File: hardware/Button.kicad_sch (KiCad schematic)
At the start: 12 parts, among them J13 Conn_01x05_Pin, J5 Conn_01x05_Pin, Q1 2N7002, Q10 2N7002, Q2 2N7002, Q3 2N7002, Q9 2N7002

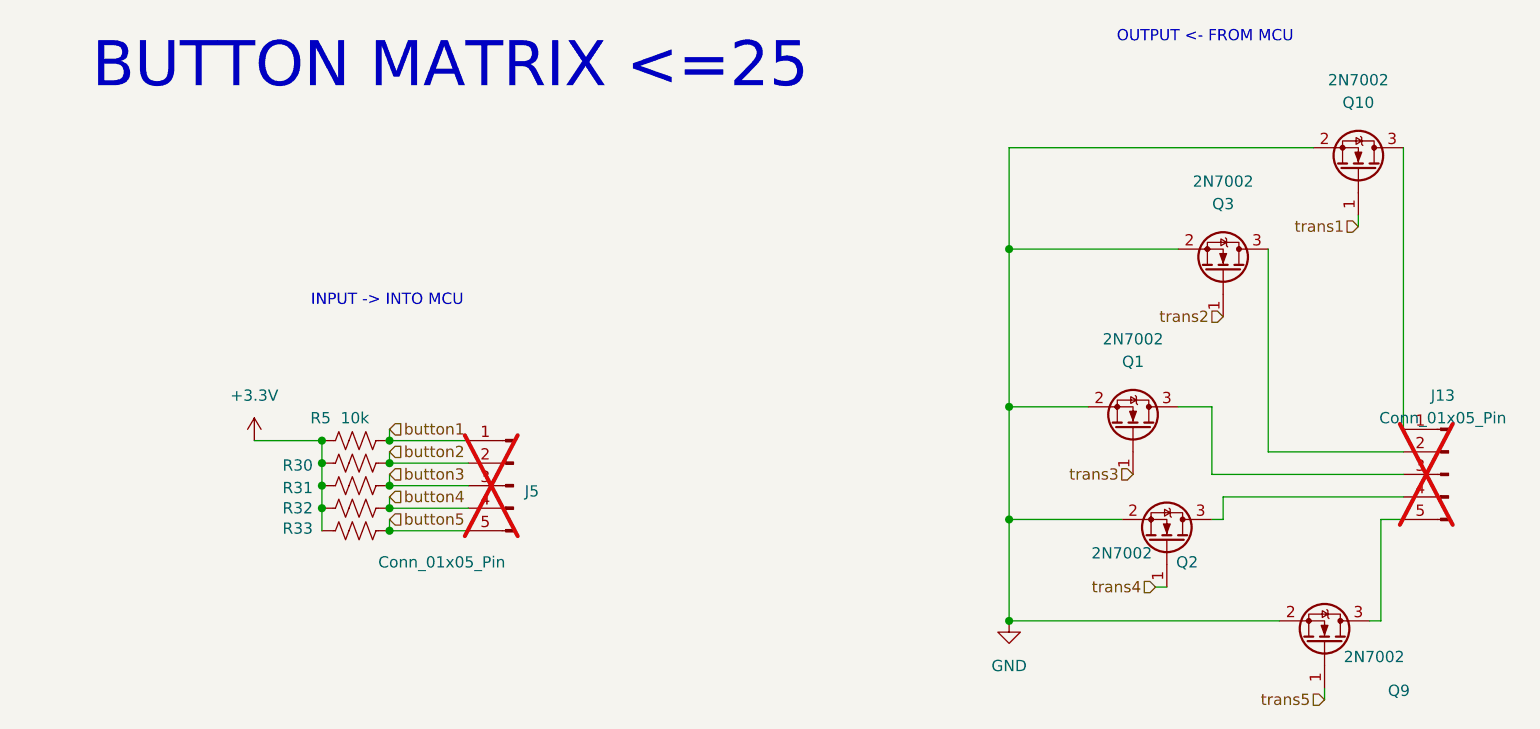
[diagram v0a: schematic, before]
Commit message: Stylistic changes
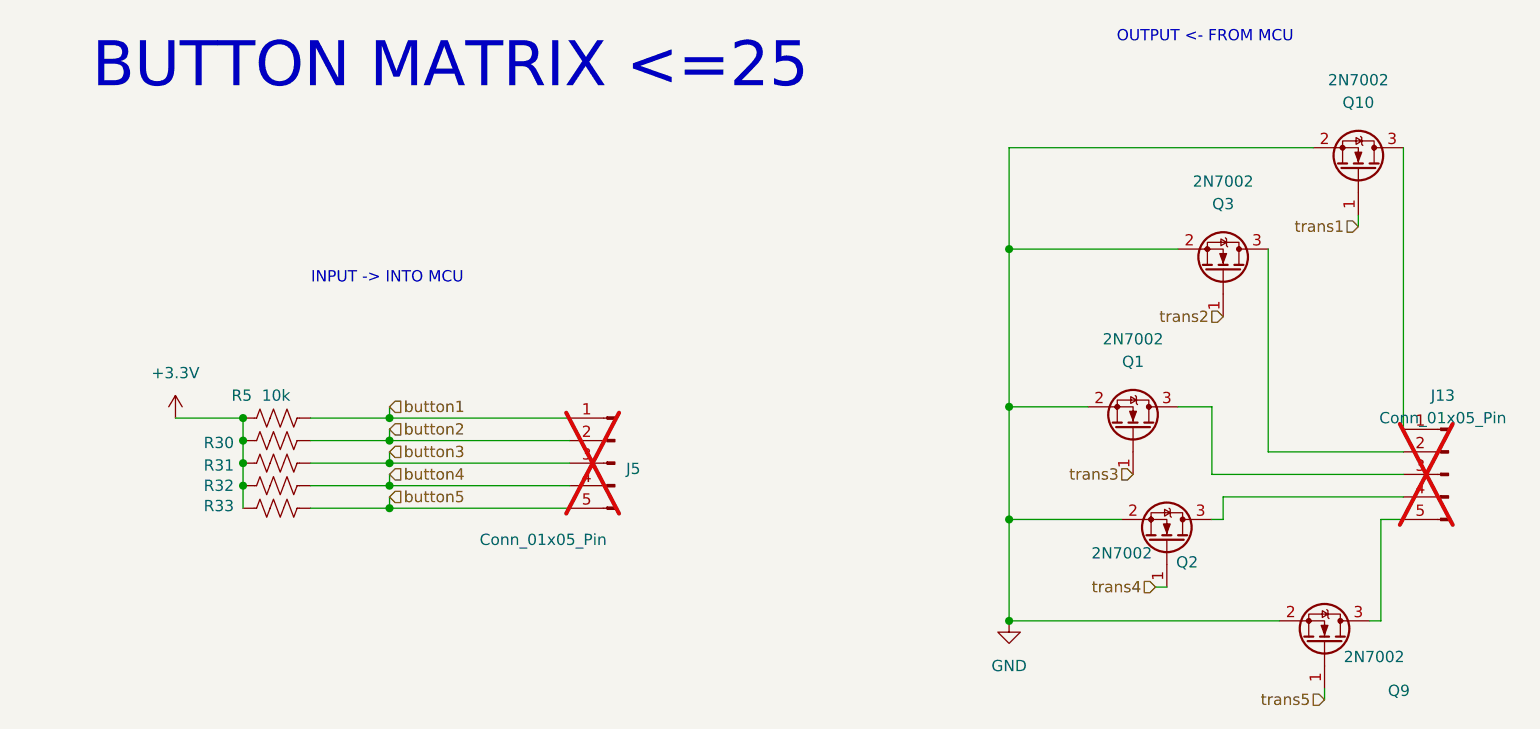
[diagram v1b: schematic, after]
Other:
- moved on the sheet: J5, R30, R31, R32, R33, R5
